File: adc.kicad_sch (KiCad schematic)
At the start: 45 parts, among them J10 Conn_01x02_Pin, J11 Conn_01x02_Pin, J12 Conn_01x02_Pin, J14 Conn_01x02_Pin, J4 Conn_01x03_Pin, J5 Conn_01x03_Pin, J8 Conn_01x03_Pin, J9 Conn_01x03_Pin, U9 LTC2299xUP

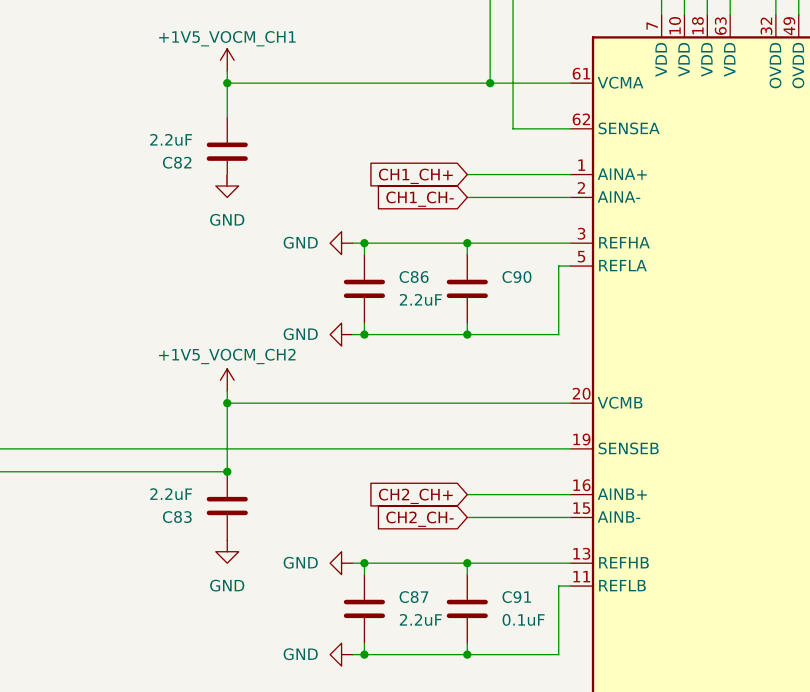
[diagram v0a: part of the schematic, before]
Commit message: Save work before adding symetrical op amp
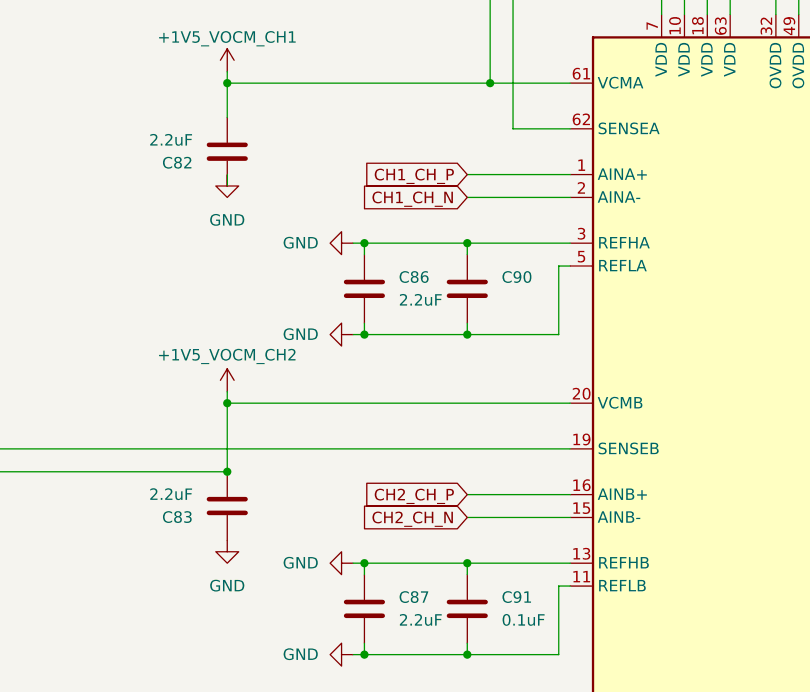
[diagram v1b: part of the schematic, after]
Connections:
- net CH1_CH+ renamed CH1_CH_P
- net CH1_CH- renamed CH1_CH_N
- net CH2_CH+ renamed CH2_CH_P
- net CH2_CH- renamed CH2_CH_N
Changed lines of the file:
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@@
 		)
 	)
-	(global_label "CH2_CH-"
+	(global_label "CH2_CH_N"
 		(shape input)
 		(at 203.2 186.69 180)
@@
 		)
 		(property "Intersheetrefs" "${INTERSHEET_REFS}"
-			(at 191.2643 186.69 0)
+			(at 190.5386 186.69 0)
 			(effects
 				(font
@@
 		)
 	)
-	(global_label "CH1_CH+"
+	(global_label "CH1_CH_P"
 		(shape input)
 		(at 203.2 148.59 180)
@@
 		)
 		(property "Intersheetrefs" "${INTERSHEET_REFS}"
-			(at 191.2643 148.59 0)
+			(at 190.5991 148.59 0)
 			(effects
 				(font
@@
 		)
 	)
-	(global_label "CH1_CH-"
+	(global_label "CH1_CH_N"
 		(shape input)
 		(at 203.2 151.13 180)
@@
 		)
 		(property "Intersheetrefs" "${INTERSHEET_REFS}"
-			(at 191.2643 151.13 0)
+			(at 190.5386 151.13 0)
 			(effects
 				(font
@@
 		)
 	)
-	(global_label "CH2_CH+"
+	(global_label "CH2_CH_P"
 		(shape input)
 		(at 203.2 184.15 180)
@@
 		)
 		(property "Intersheetrefs" "${INTERSHEET_REFS}"
-			(at 191.2643 184.15 0)
+			(at 190.5991 184.15 0)
 			(effects
 				(font
